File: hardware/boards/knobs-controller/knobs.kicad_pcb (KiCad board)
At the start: 2 copper layers, 110.5 x 111.1 mm, 175 parts, among them J1 ZX62-AB-5PA(31), J10 Conn_01x01_Female, J11 Conn_01x01_Female, J12 Conn_01x01_Female, J13 Conn_01x01_Female, J14 Conn_01x01_Female, J15 Conn_01x01_Female, J16 Conn_01x01_Female, J17 Conn_01x01_Female, J18 Conn_01x01_Female, J19 Conn_01x01_Female, J2 2X3_SMD_MALE, J20 Conn_01x01_Female, J21 Conn_01x01_Female, J22 Conn_01x01_Female, J23 Conn_01x01_Female, J24 Conn_01x01_Female, J25 Conn_01x01_Female, J26 Conn_01x01_Female, J27 Conn_01x01_Female, J28 Conn_01x01_Female, J29 Conn_01x01_Female, J3 Conn_01x01_Female, J30 Conn_01x01_Female, J31 Conn_01x01_Female, J32 Conn_01x01_Female, J33 Conn_01x01_Female, J34 Conn_01x01_Female, J35 Conn_01x01_Female, J36 Conn_01x01_Female, J37 Conn_01x01_Female, J38 Conn_01x01_Female, J39 Conn_01x01_Female, J4 Conn_01x01_Female, J40 Conn_01x01_Female, J41 Conn_01x01_Female, J42 Conn_01x01_Female, J43 Conn_01x01_Female, J44 Conn_01x01_Female, J45 Conn_01x01_Female, J46 Conn_01x01_Female, J47 Conn_01x01_Female, J48 Conn_01x01_Female, J49 Conn_01x01_Female, J5 Conn_01x01_Female, J50 Conn_01x01_Female, J51 Conn_01x01_Female, J52 Conn_01x01_Female, J53 Conn_01x01_Female, J54 Conn_01x01_Female, J55 Conn_01x01_Female, J56 Conn_01x01_Female, J57 WURTH_ELECTRONICS_61400413321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, J58 USB-A-S-X-X-VT, J59 ST7735_1.4, J6 Conn_01x01_Female, J7 Conn_01x01_Female, J8 Conn_01x01_Female, J9 Conn_01x01_Female, SW1 Rotary Encoder, SW2 Rotary Encoder, SW3 Rotary Encoder, U1 ATSAMD21G18A-48, U2 AP7215-33YG-13, U3 ANALOG_DEVICES_AD7606BSTZANAL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, U4 ANALOG_DEVICES_AD5754BREZANAL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, U5 MICROCHIP_MCP1700T-2502E-TTMI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, Y1 32.768KHz

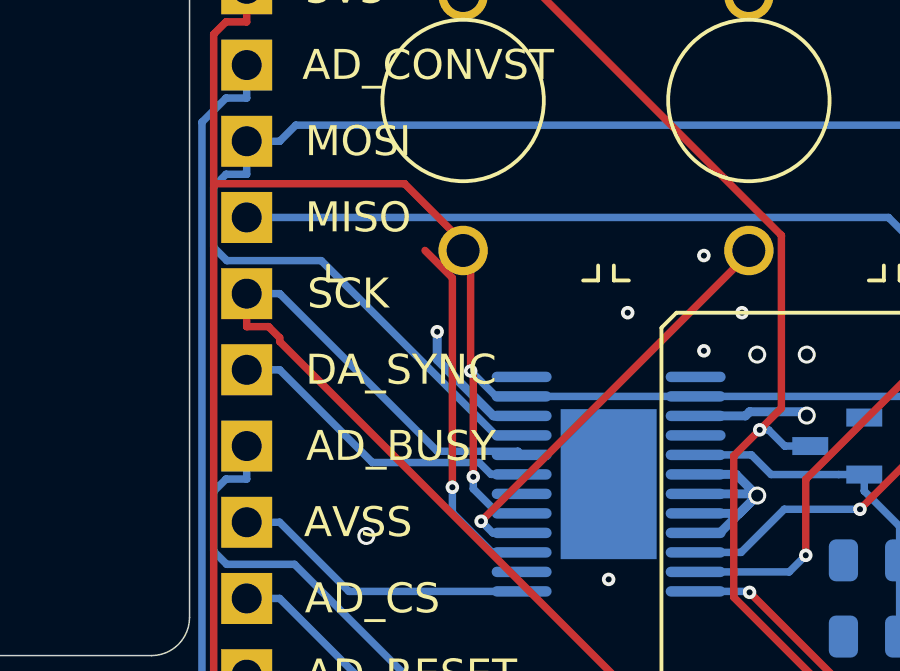
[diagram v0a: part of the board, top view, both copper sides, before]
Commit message: knobs v1.7 finalisation
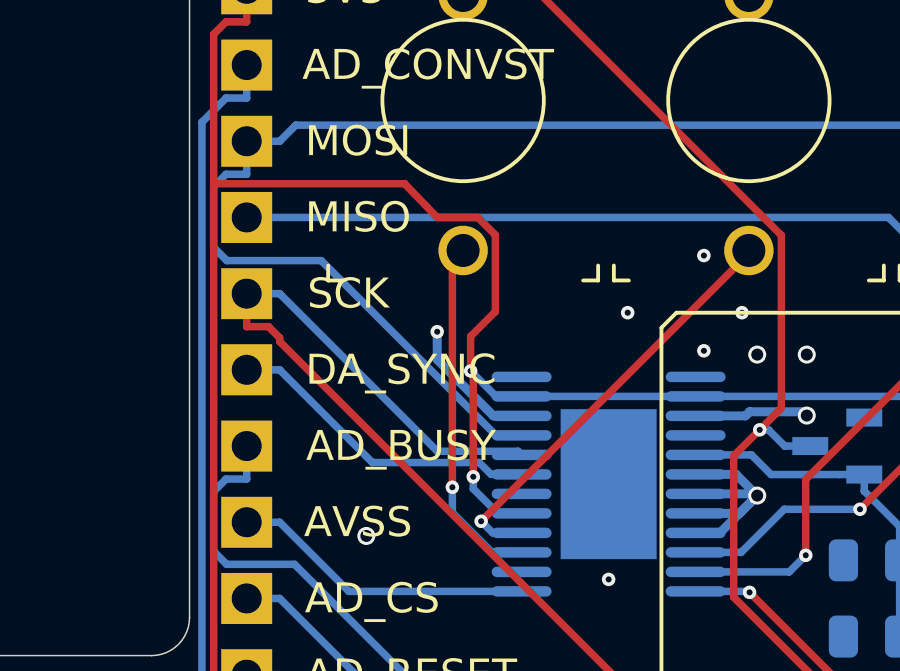
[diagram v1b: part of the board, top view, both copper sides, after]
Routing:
- net +3V3: track 542.6 -> 544.0 mm
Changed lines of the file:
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@@
     (thickness 1.6)
     (drawings 316)
-    (tracks 1356)
+    (tracks 1360)
     (zones 0)
     (modules 175)
@@
   (segment (start 121.8012 96.1962) (end 123.38 97.775) (width 0.25) (layer Top) (net 45))
   (segment (start 107.0478 96.1962) (end 121.8012 96.1962) (width 0.25) (layer Top) (net 45))
-  (segment (start 114.1446 64.5767) (end 114.1446 68.6183) (width 0.25) (layer Top) (net 45))
-  (segment (start 111.9446 62.3767) (end 114.1446 64.5767) (width 0.25) (layer Top) (net 45))
   (segment (start 105.5797 62.3767) (end 111.9446 62.3767) (width 0.25) (layer Top) (net 45))
   (segment (start 105.5797 57.3929) (end 105.5797 62.3767) (width 0.25) (layer Top) (net 45))
@@
   (segment (start 165.4903 123.0417) (end 172.4525 123.0417) (width 0.25) (layer Top) (net 45))
   (segment (start 174.9904 118.7954) (end 173.99 117.795) (width 0.25) (layer Top) (net 45))
+  (segment (start 114.384002 63.5) (end 113.03 63.5) (width 0.25) (layer Top) (net 45))
+  (segment (start 114.969001 64.084999) (end 114.384002 63.5) (width 0.25) (layer Top) (net 45))
+  (segment (start 114.969001 66.640999) (end 114.969001 64.084999) (width 0.25) (layer Top) (net 45))
+  (segment (start 114.1446 67.4654) (end 114.969001 66.640999) (width 0.25) (layer Top) (net 45))
+  (segment (start 111.9446 62.3767) (end 113.03 63.5) (width 0.25) (layer Top) (net 45))
+  (segment (start 114.1446 67.4654) (end 114.1446 68.6183) (width 0.25) (layer Top) (net 45))
   (via (at 127.3435 118.1913) (size 0.45) (layers Top Bottom) (net 46))
   (via (at 135.1722 101.2693) (size 0.45) (layers Top Bottom) (net 46))
@@
   (segment (start 114.4945 73.6269) (end 123.419 64.7024) (width 0.25) (layer Top) (net 88))
   (via (at 113.5352 72.4934) (size 0.45) (layers Top Bottom) (net 89))
-  (segment (start 113.5352 65.5122) (end 112.624 64.601) (width 0.25) (layer Top) (net 89))
-  (segment (start 113.5352 72.4934) (end 113.5352 65.5122) (width 0.25) (layer Top) (net 89))
   (segment (start 114.8605 74.665) (end 115.845 74.665) (width 0.25) (layer Bottom) (net 89))
   (segment (start 113.5353 73.3398) (end 114.8605 74.665) (width 0.25) (layer Bottom) (net 89))
   (segment (start 113.5353 72.4934) (end 113.5353 73.3398) (width 0.25) (layer Bottom) (net 89))
   (segment (start 113.5352 72.4934) (end 113.5353 72.4934) (width 0.25) (layer Bottom) (net 89))
+  (segment (start 113.5352 64.9598) (end 113.766278 64.728722) (width 0.25) (layer Top) (net 89))
+  (segment (start 113.5352 72.4934) (end 113.5352 64.9598) (width 0.25) (layer Top) (net 89))
   (via (at 120.6798 40.0285) (size 0.45) (layers Top Bottom) (net 90))
   (segment (start 122.1951 38.5132) (end 120.6798 40.0285) (width 0.25) (layer Bottom) (net 90))
